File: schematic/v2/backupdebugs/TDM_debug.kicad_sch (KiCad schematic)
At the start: 16 parts, among them J23 USB_A, J4 TDM_DBG, U34 CH340G, Y3 Crystal

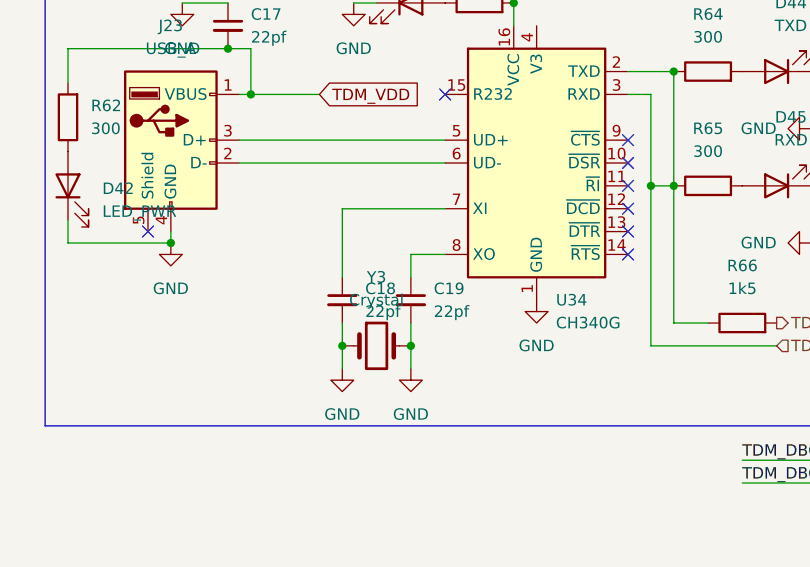
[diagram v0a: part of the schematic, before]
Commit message: time to start routing?
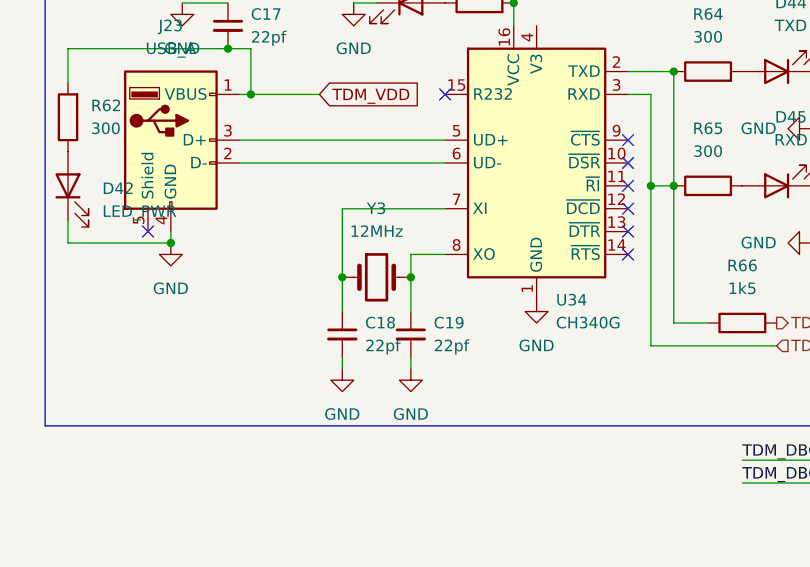
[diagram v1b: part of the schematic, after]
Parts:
- Y3: value Crystal -> 12MHz; footprint (none) -> Crystal:Crystal_C26-LF_D2.1mm_L6.5mm_Horizontal
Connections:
- net GND: no longer Y3.1, Y3.2
- net at C19.1, U34.8 (XO): now also Y3.2
- net at C18.1, U34.7 (XI): now also Y3.1
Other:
- moved on the sheet: C18, C19
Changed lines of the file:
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@@
+	)
+	(junction
+		(at 116.84 73.66)
+		(diameter 0)
+		(color 0 0 0 0)
 	)
 	(junction
@@
 	)
 	(junction
-		(at 116.84 81.28)
-		(diameter 0)
-		(color 0 0 0 0)
-	)
-	(junction
 		(at 90.17 69.85)
 		(diameter 0)
@@
 	)
 	(junction
-		(at 109.22 81.28)
-		(diameter 0)
-		(color 0 0 0 0)
-	)
-	(junction
 		(at 146.05 63.5)
 		(diameter 0)
 		(color 0 0 0 0)
 	)
+	(junction
+		(at 109.22 73.66)
+		(diameter 0)
+		(color 0 0 0 0)
+	)
 	(no_connect
 		(at 140.97 68.58)
@@
 	(wire
 		(pts
+			(xy 116.84 73.66) (xy 116.84 77.47)
+		)
+		(stroke
+			(width 0)
+			(type default)
+		)
+	)
+	(wire
+		(pts
 			(xy 99.06 53.34) (xy 106.68 53.34)
 		)
@@
 	(wire
 		(pts
-			(xy 109.22 83.82) (xy 109.22 81.28)
+			(xy 109.22 82.55) (xy 109.22 83.82)
 		)
 		(stroke
@@
 	(wire
 		(pts
-			(xy 109.22 78.74) (xy 109.22 81.28)
-		)
-		(stroke
-			(width 0)
-			(type default)
-		)
-	)
-	(wire
-		(pts
 			(xy 90.17 69.85) (xy 78.74 69.85)
 		)
@@
 	(wire
 		(pts
-			(xy 116.84 78.74) (xy 116.84 81.28)
-		)
-		(stroke
-			(width 0)
-			(type default)
-		)
-	)
-	(wire
-		(pts
-			(xy 116.84 81.28) (xy 116.84 83.82)
+			(xy 116.84 82.55) (xy 116.84 83.82)
 		)
 		(stroke
@@
 		(pts
 			(xy 146.05 63.5) (xy 146.05 78.74)
+		)
+		(stroke
+			(width 0)
+			(type default)
+		)
+	)
+	(wire
+		(pts
+			(xy 109.22 73.66) (xy 109.22 77.47)
 		)
 		(stroke
@@
 	)
 	(symbol
+		(lib_id "Device:Crystal")
+		(at 113.03 73.66 0)
+		(unit 1)
+		(exclude_from_sim no)
+		(in_bom yes)
+		(on_board yes)
+		(dnp no)
+		(fields_autoplaced yes)
+		(property "Reference" "Y3"
+			(at 113.03 66.04 0)
+			(effects
+				(font
+					(size 1.27 1.27)
+				)
+			)
+		)
+		(property "Value" "12MHz"
+			(at 113.03 68.58 0)
+			(effects
+				(font
+					(size 1.27 1.27)
+				)
+			)
+		)
+		(property "Footprint" "Crystal:Crystal_C26-LF_D2.1mm_L6.5mm_Horizontal"
+			(at 113.03 73.66 0)
+			(effects
+				(font
+					(size 1.27 1.27)
+				)
+				(hide yes)
+			)
+		)
+		(property "Datasheet" "~"
+			(at 113.03 73.66 0)
+			(effects
+				(font
+					(size 1.27 1.27)
+				)
+				(hide yes)
+			)
+		)
+		(property "Description" "Two pin crystal"
+			(at 113.03 73.66 0)
+			(effects
+				(font
+					(size 1.27 1.27)
+				)
+				(hide yes)
+			)
+		)
+		(pin "1"
+		)
+		(pin "2"
+		)
+		(instances
+			(project "signalmesh"
+				(path "/fe7b15e9-f0ed-4338-9f03-dd7651dace13/442c7b41-f8c0-48e5-8b80-63d502cac366/3e15aa38-e071-402c-a18d-97def628e870"
+					(reference "Y3")
+					(unit 1)
+				)
+			)
+		)
+	)
+	(symbol
 		(lib_id "Device:LED")
 		(at 157.48 50.8 180)
@@
 	(symbol
 		(lib_id "Device:C_Small")
-		(at 116.84 76.2 0)
+		(at 116.84 80.01 0)
 		(unit 1)
 		(exclude_from_sim no)
@@
 		(fields_autoplaced yes)
 		(property "Reference" "C19"
-			(at 119.38 74.9362 0)
+			(at 119.38 78.7462 0)
 			(effects
 				(font
@@
 		)
 		(property "Value" "22pf"
-			(at 119.38 77.4762 0)
+			(at 119.38 81.2862 0)
 			(effects
 				(font
@@
 		)
 		(property "Footprint" "Capacitor_SMD:C_0805_2012Metric"
-			(at 116.84 76.2 0)
+			(at 116.84 80.01 0)
 			(effects
 				(font
@@
 		)
 		(property "Datasheet" "~"
-			(at 116.84 76.2 0)
+			(at 116.84 80.01 0)
 			(effects
 				(font
@@
 		)
 		(property "Description" "Unpolarized capacitor, small symbol"
-			(at 116.84 76.2 0)
+			(at 116.84 80.01 0)
 			(effects
 				(font
@@
 	)
 	(symbol
-		(lib_id "Device:Crystal")
-		(at 113.03 81.28 0)
-		(unit 1)
-		(exclude_from_sim no)
-		(in_bom yes)
-		(on_board yes)
-		(dnp no)
-		(fields_autoplaced yes)
-		(property "Reference" "Y3"
-			(at 113.03 73.66 0)
-			(effects
-				(font
-					(size 1.27 1.27)
-				)
-			)
-		)
-		(property "Value" "Crystal"
-			(at 113.03 76.2 0)
-			(effects
-				(font
-					(size 1.27 1.27)
-				)
-			)
-		)
-		(property "Footprint" ""
-			(at 113.03 81.28 0)
-			(effects
-				(font
-					(size 1.27 1.27)
-				)
-				(hide yes)
-			)
-		)
-		(property "Datasheet" "~"
-			(at 113.03 81.28 0)
-			(effects
-				(font
-					(size 1.27 1.27)
-				)
-				(hide yes)
-			)
-		)
-		(property "Description" "Two pin crystal"
-			(at 113.03 81.28 0)
-			(effects
-				(font
-					(size 1.27 1.27)
-				)
-				(hide yes)
-			)
-		)
-		(pin "1"
-		)
-		(pin "2"
-		)
-		(instances
-			(project "signalmesh"
-				(path "/fe7b15e9-f0ed-4338-9f03-dd7651dace13/442c7b41-f8c0-48e5-8b80-63d502cac366/3e15aa38-e071-402c-a18d-97def628e870"
-					(reference "Y3")
-					(unit 1)
-				)
-			)
-		)
-	)
-	(symbol
 		(lib_id "Device:C_Small")
 		(at 96.52 45.72 0)
@@
 	(symbol
 		(lib_id "Device:C_Small")
-		(at 109.22 76.2 0)
+		(at 109.22 80.01 0)
 		(unit 1)
 		(exclude_from_sim no)
@@
 		(fields_autoplaced yes)
 		(property "Reference" "C18"
-			(at 111.76 74.9362 0)
+			(at 111.76 78.7462 0)
 			(effects
 				(font
@@
 		)
 		(property "Value" "22pf"
-			(at 111.76 77.4762 0)
+			(at 111.76 81.2862 0)
 			(effects
 				(font
@@
 		)
 		(property "Footprint" "Capacitor_SMD:C_0805_2012Metric"
-			(at 109.22 76.2 0)
+			(at 109.22 80.01 0)
 			(effects
 				(font
@@
 		)
 		(property "Datasheet" "~"
-			(at 109.22 76.2 0)
+			(at 109.22 80.01 0)
 			(effects
 				(font
@@
 		)
 		(property "Description" "Unpolarized capacitor, small symbol"
-			(at 109.22 76.2 0)
-			(effects
-				(font
+			(at 109.22 80.01 0)
+			(effects
+				(font
